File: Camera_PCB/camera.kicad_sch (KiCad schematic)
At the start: 19 parts, among them J1 1-84952-5, J2 USB_A, Y2 Crystal_GND3, Y4 Crystal_GND24

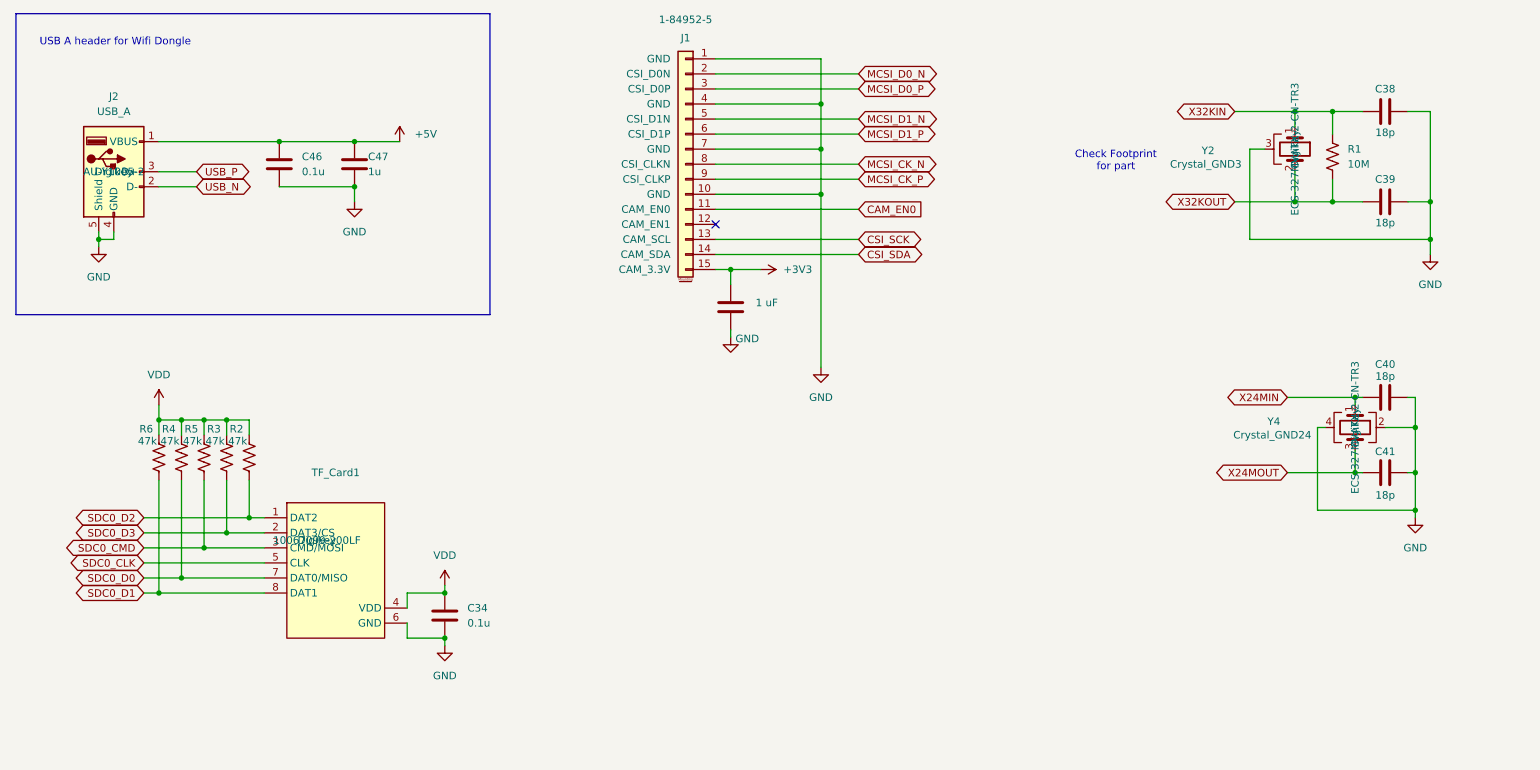
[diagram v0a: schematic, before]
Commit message: Camera PCB Schematic review 1
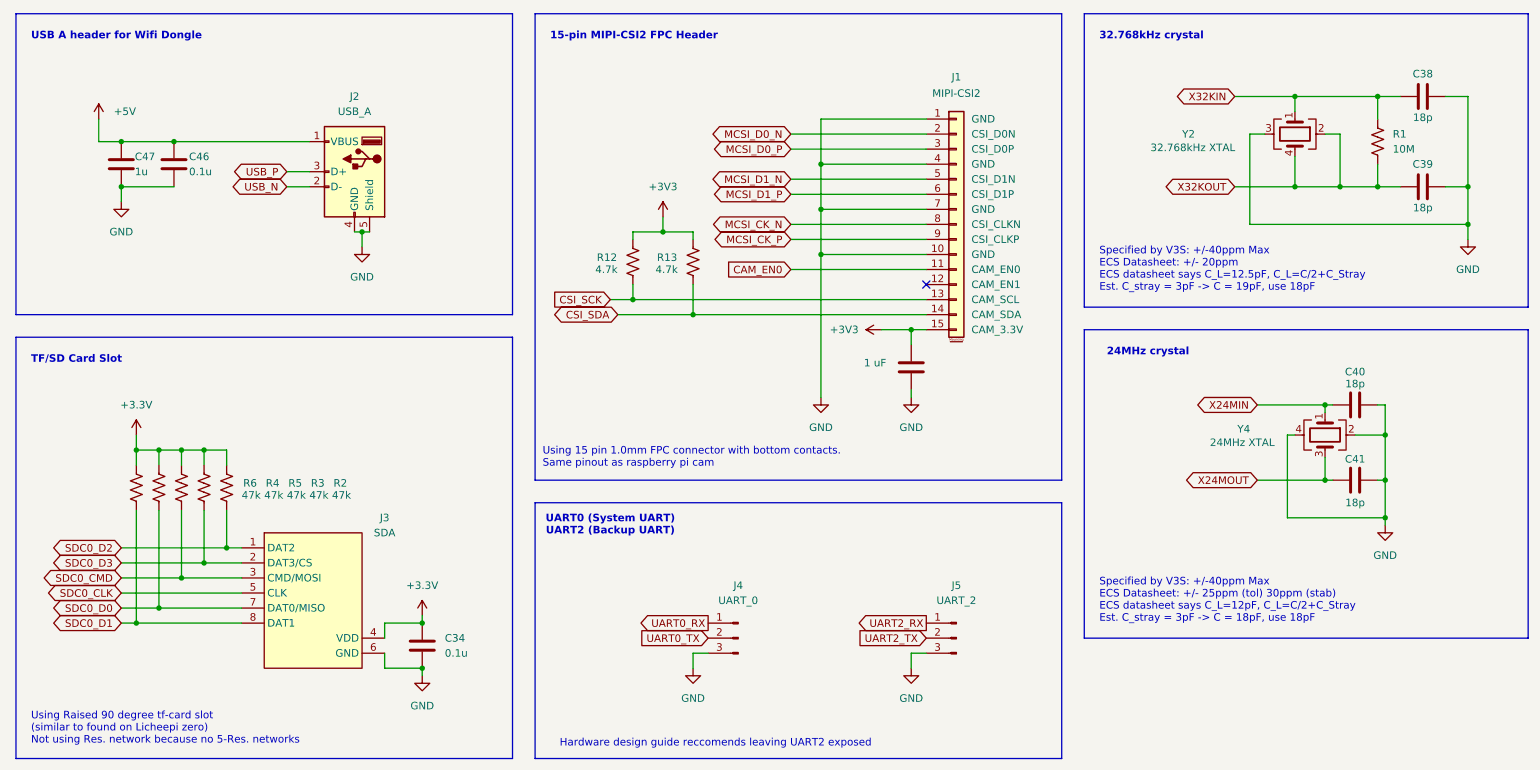
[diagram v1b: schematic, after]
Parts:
- added J4: UART_0, Connector_PinHeader_2.54mm:PinHeader_1x03_P2.54mm_Vertical, symbol Connector:Conn_01x03_Pin
- added J5: UART_2, Connector_PinHeader_2.54mm:PinHeader_1x03_P2.54mm_Vertical, symbol Connector:Conn_01x03_Pin
- added R12, R13: 4.7k, Resistor_SMD:R_0805_2012Metric_Pad1.20x1.40mm_HandSolder, symbol Device:R_US
- J1: value 1-84952-5 -> MIPI-CSI2; DPN (none) -> 1-84952-5; Distributor (none) -> DigiKey
- J2: footprint Connector_USB:USB_A_Connfly_DS1095 -> Connector_USB:USB_A_Receptacle_GCT_USB1046; DPN AU-Y1005-2 -> USB1046-GF-0190-L-B-A; Distributor Digikey -> DigiKey
- J3: renamed from TF_Card1; value ~ -> SDA; Distributor Digikey -> DigiKey
- R1: footprint Resistor_SMD:R_0805_2012Metric_Pad1.20x1.40mm_HandSolder -> Resistor_SMD:R_0603_1608Metric_Pad0.98x0.95mm_HandSolder
- Y2: value Crystal_GND3 -> 32.768kHz XTAL; footprint BackupCamCustomParts:OSC_ECS-2520S25-250-FN-TR -> BackupCamCustomParts:XTAL_ECS-.327-12.5-38-TR; symbol Device:Crystal_GND3 -> Device:Crystal_GND23; DPN ECS-327MVATX-2-CN-TR3 -> ECS-.327-12.5-38-TR
- Y4: value Crystal_GND24 -> 24MHz XTAL; footprint BackupCamCustomParts:OSC_ECS-2520S25-250-FN-TR -> BackupCamCustomParts:XTAL_ECS-240-12-36-AGN-TR; DPN ECS-327MVATX-2-CN-TR3 -> ECS-240-12-36-AGN-TR
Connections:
- net +3V3: now also R12.1, R13.1
- net CSI_SCK: now also R12.2
- net CSI_SDA: now also R13.2
- net GND: now also J4.3 (Pin_3), J5.3 (Pin_3)
- net X32KOUT: now also Y2.4
- net VDD renamed +3.3V
- new net UART0_RX: J4.1 (Pin_1)
- new net UART0_TX: J4.2 (Pin_2)
- new net UART2_RX: J5.1 (Pin_1)
- new net UART2_TX: J5.2 (Pin_2)
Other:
- note added: "15-pin MIPI-CSI2 FPC Header"
- note added: "24MHz crystal"
- note added: "32.768kHz crystal"
- note added: "Hardware design guide reccomends leaving UART2 exposed"
- note added: "Specified by V3S: +/-40ppm Max ECS Datasheet: +/- 20ppm ECS datasheet says C_L=12.5pF, C_L=C/2+C_Stray Est. C_stray = 3pF -> C = 19pF, use 18pF"
- note added: "Specified by V3S: +/-40ppm Max ECS Datasheet: +/- 25ppm (tol) 30ppm (stab) ECS datasheet says C_L=12pF, C_L=C/2+C_Stray Est. C_stray = 3pF -> C = 18pF, use 18pF"
- note added: "TF/SD Card Slot"
- note added: "UART0 (System UART) UART2 (Backup UART)"
- note added: "Using 15 pin 1.0mm FPC connector with bottom contacts. Same pinout as raspberry pi cam"
- note added: "Using Raised 90 degree tf-card slot (similar to found on Licheepi zero) Not using Res. network because no 5-Res. networks"
- note removed: "Check Footprint for part"
- moved on the sheet: C34, C38, C39, C40, C41, C46, C47, J1, J2, J3, R1, R2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
